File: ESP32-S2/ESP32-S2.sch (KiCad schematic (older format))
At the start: 38 parts, among them J1 USB_A, J2 TYPE-C-31-M-12, J3 Conn_01x18_Male, J4 Conn_01x22_Male, Q1 L8050QLT1G, Q2 L8050QLT1G, SW1 SW_Push, SW2 SW_Push, U1 ESP32-S2-WROOM-ESP32-S2-WROOM, U2 CH340C, U3 AMS1117-3.3

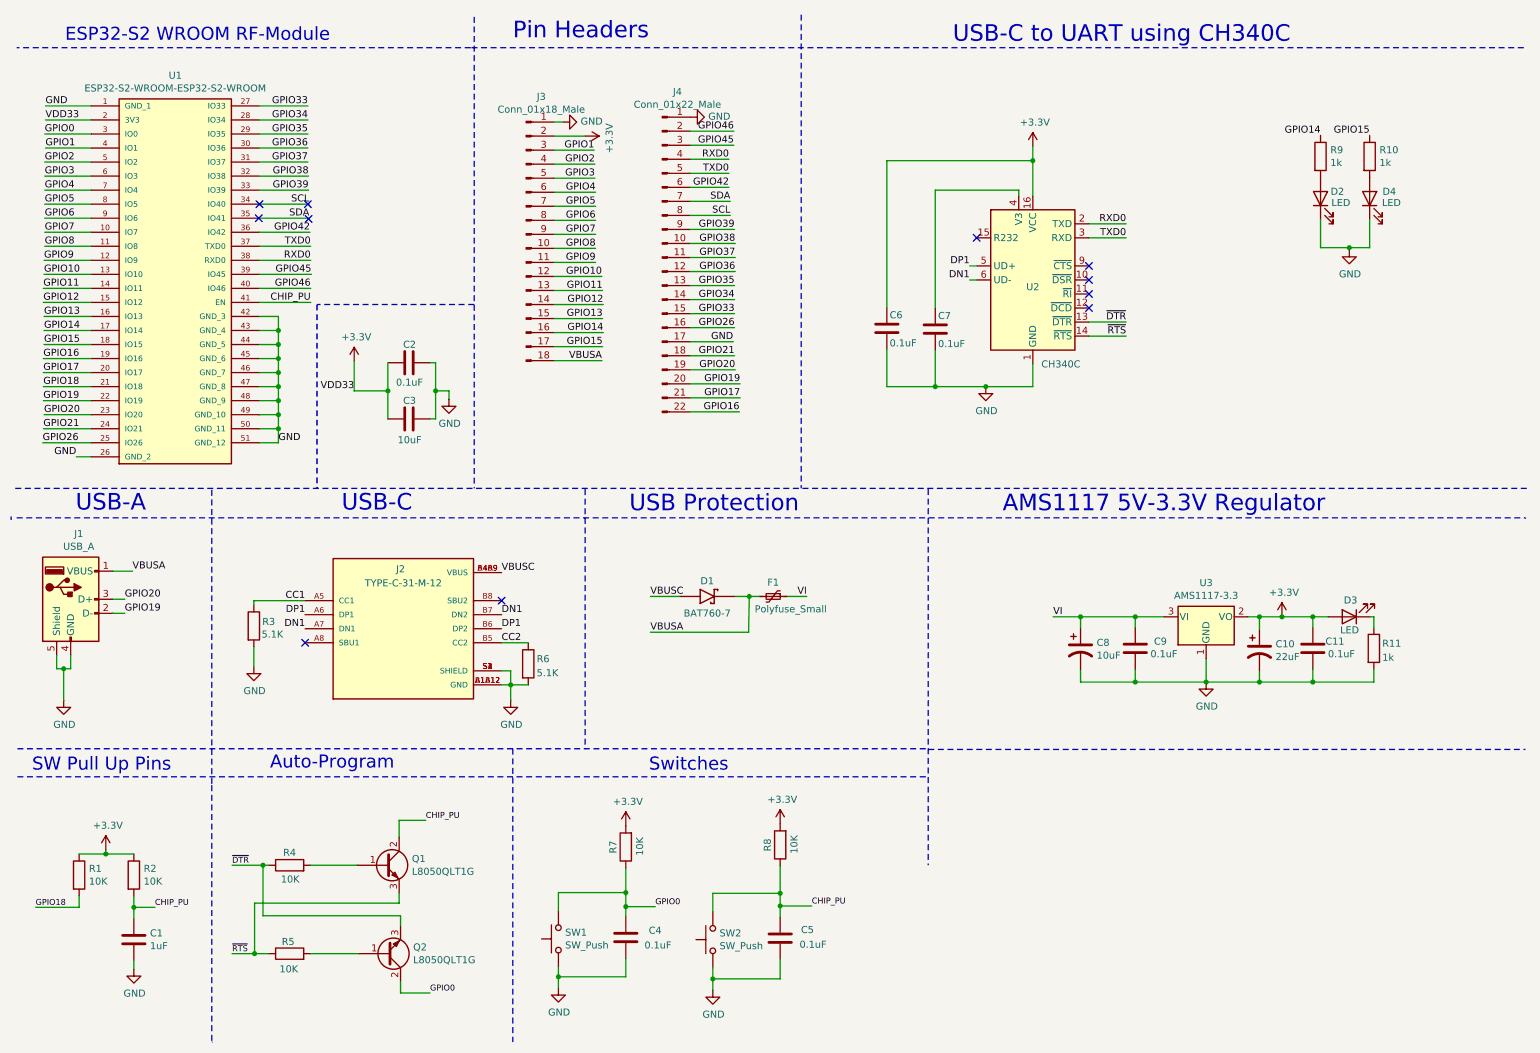
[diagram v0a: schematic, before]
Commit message: addedassets, updateed silkscreen
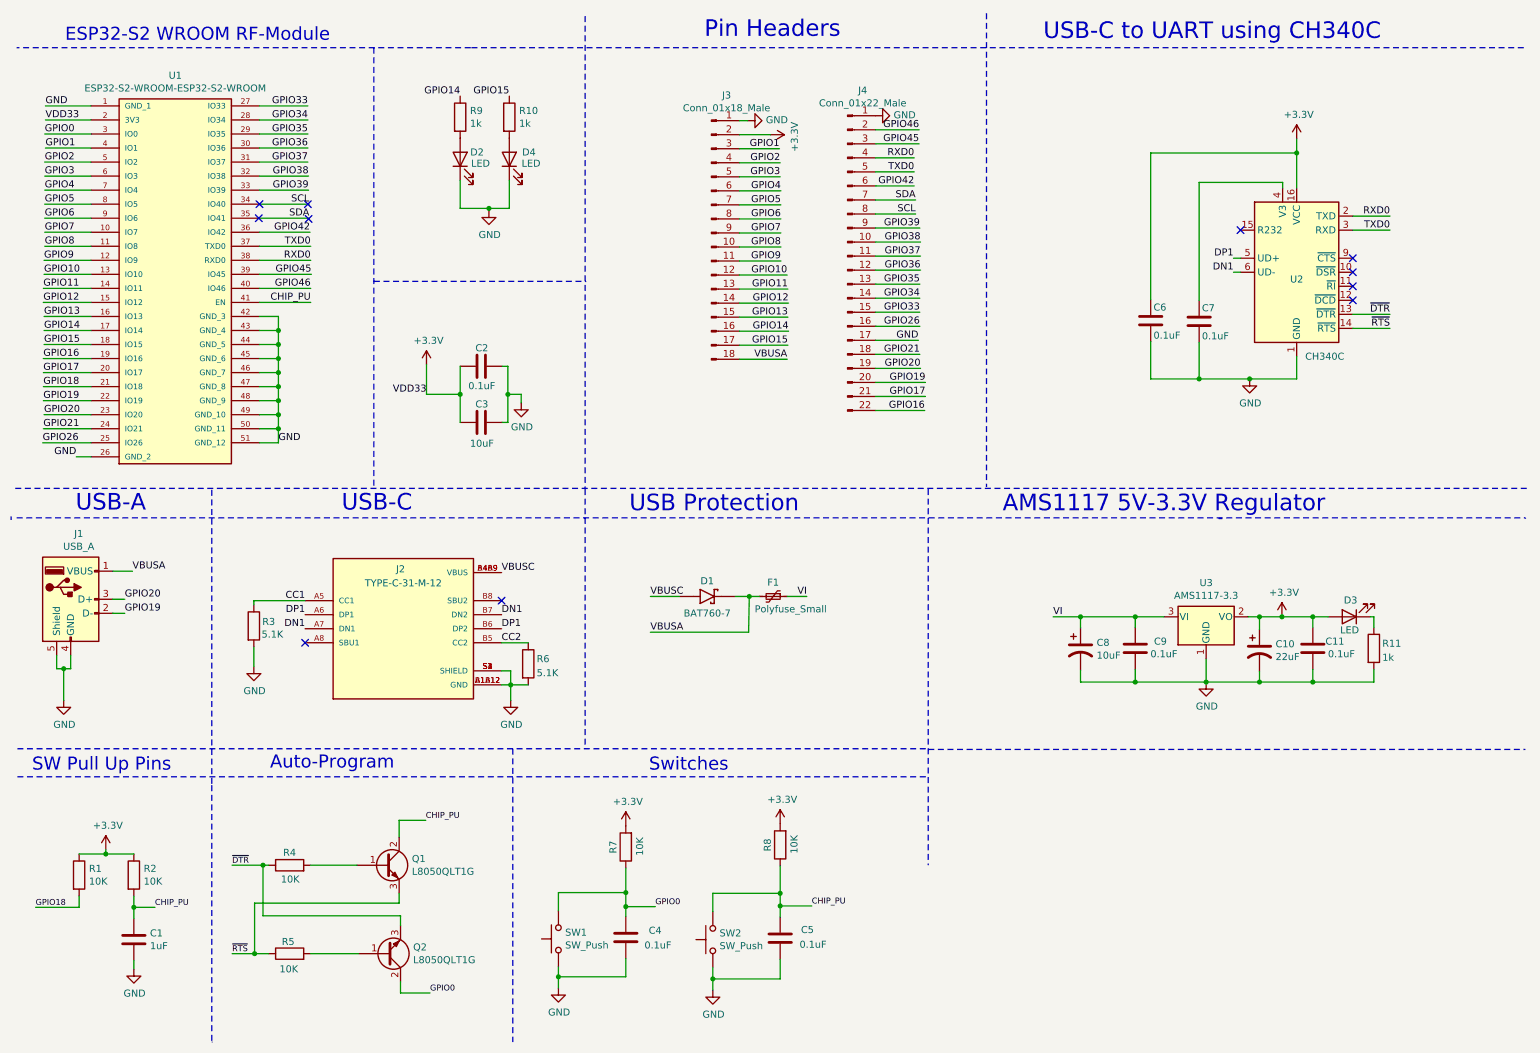
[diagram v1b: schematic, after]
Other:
- moved on the sheet: C2, C3, C6, C7, D2, D4, J3, J4, R10, R9, U2
